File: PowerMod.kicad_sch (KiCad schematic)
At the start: 7 parts, among them J1 Conn_01x12_Pin, J2 Conn_01x12_Pin, U1 L7805

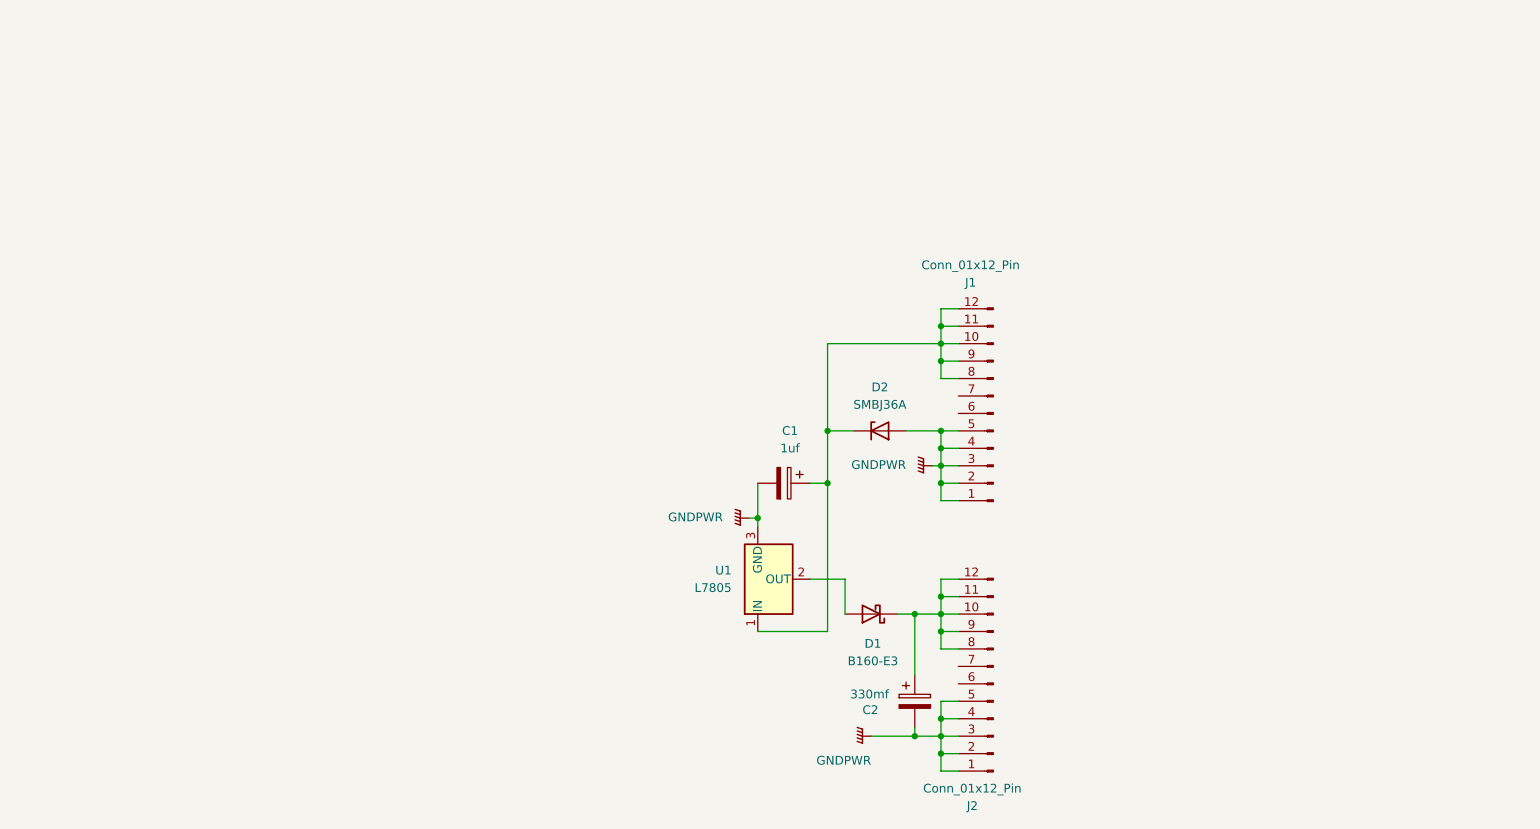
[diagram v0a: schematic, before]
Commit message: Updated schematic to be much clearer
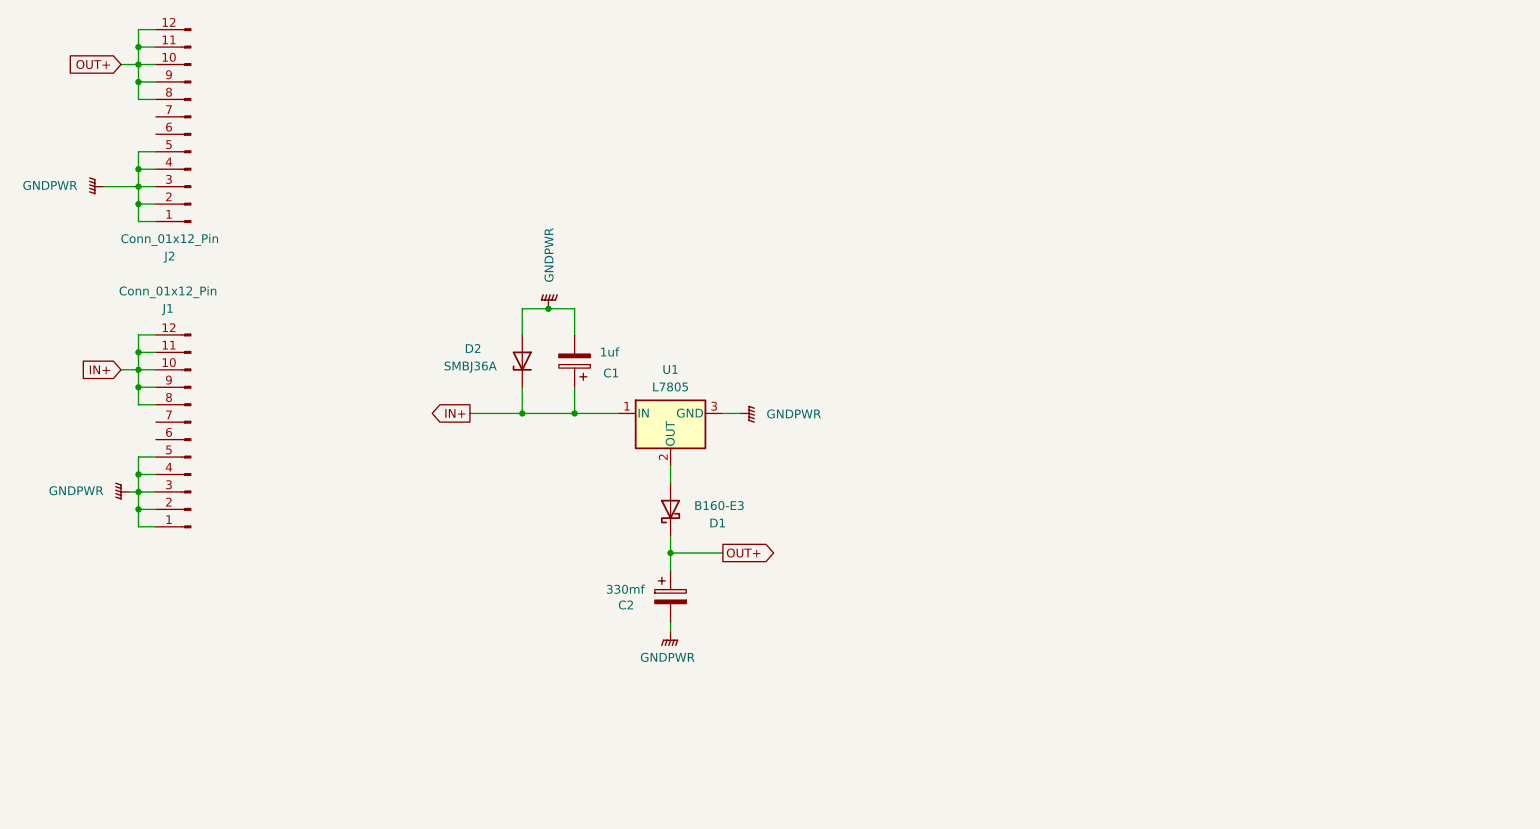
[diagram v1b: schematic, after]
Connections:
- net OUT+: now reaches C2.1, D1.1 (K), J2.10 (Pin_10), J2.11 (Pin_11), J2.12 (Pin_12), J2.8 (Pin_8), J2.9 (Pin_9)
- net IN+: now reaches C1.1, D2.1 (K), J1.10 (Pin_10), J1.11 (Pin_11), J1.12 (Pin_12), J1.8 (Pin_8), J1.9 (Pin_9), U1.1 (IN)
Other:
- moved on the sheet: C1, C2, D1, D2, J1, J2, U1

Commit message: Complete re-design
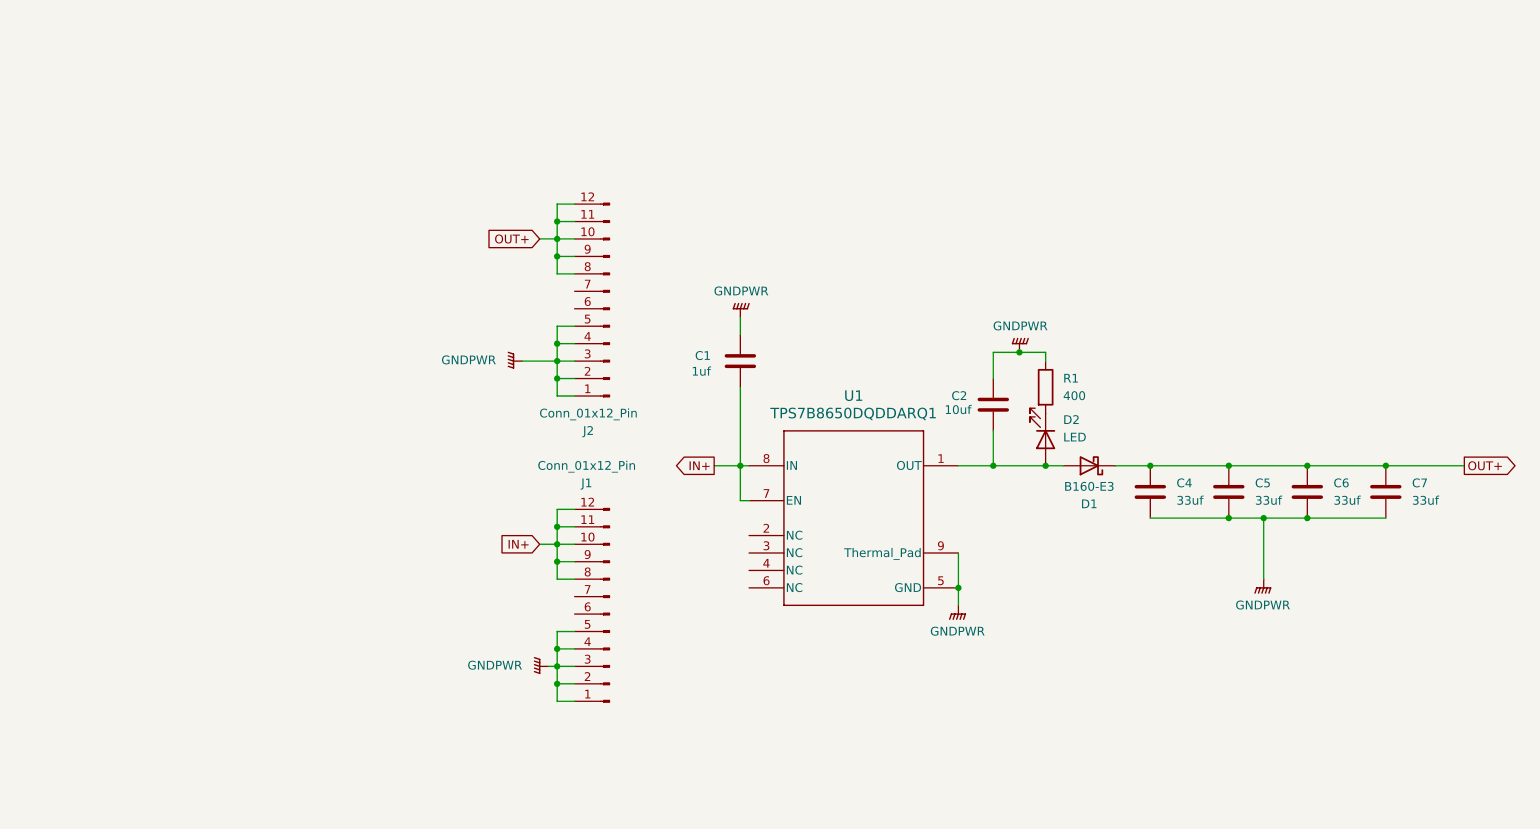
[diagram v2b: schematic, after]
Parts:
- removed C1: 1uf, Custom:CAPMP3.7X2.8_2.1N_KEM, symbol Device:C_Polarized
- removed C2: 330mf, Custom:CAP_20SVPK68M, symbol Device:C_Polarized
- removed D1: B160-E3, Diode_SMD:D_SMA, symbol Diode:B160-E3
- removed D2: SMBJ36A, Custom:DIOM4336X265N, symbol Device:D_Zener
- removed U1: L7805, Custom:VREG_L7805CDT-TR, symbol Regulator_Linear:L7805
- added C1: 1uf, Capacitor_SMD:C_1206_3216Metric, symbol SymbolLib2:C
- added C2: 10uf, Capacitor_SMD:C_1206_3216Metric, symbol SymbolLib2:C
- added C4, C5, C6, C7: 33uf, Capacitor_SMD:C_1206_3216Metric, symbol SymbolLib2:C
- added D1: B160-E3, Diode_SMD:D_SMA, symbol SymbolLib2:B160-E3
- added D2: LED, LED_SMD:LED_0805_2012Metric, symbol SymbolLib2:LED
- added R1: 400, Resistor_SMD:R_1206_3216Metric, symbol SymbolLib2:R
- added U1: TPS7B8650DQDDARQ1, Footprints:DDA0008B-IPC_B, symbol SymbolLib2:TPS7B8650DQDDARQ1
- J1, J2: symbol Connector:Conn_01x12_Pin -> SymbolLib2:Conn_01x12_Pin
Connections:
- net GNDPWR: now also C1.1, C2.1, C4.2, C5.2, C6.2, C7.2, R1.1, U1.5 (GND), U1.9 (Thermal_Pad)
- net IN+: now also C1.2, U1.7 (EN), U1.8 (IN)
- net OUT+: now also C4.1, C5.1, C6.1, C7.1, D1.1 (K)
- new net: C2.2, D1.2 (A), D2.2 (A), U1.1 (OUT)
- new net: D2.1 (K), R1.2
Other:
- moved on the sheet: J1, J2
